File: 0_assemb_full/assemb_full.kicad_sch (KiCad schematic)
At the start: 19 parts, among them J1 BarrelJack, J11 OutToRPi, J2 Conn_02x06, J3 AudioJack3, J4 Servo0Conn_01x03, J5 Servo1Conn_01x03, J6 Servo2Conn_01x03, J7 Servo3Conn_01x03, J8 Servo4Conn_01x03, U1 LM2902, U2 LD1117S33TR_SOT223

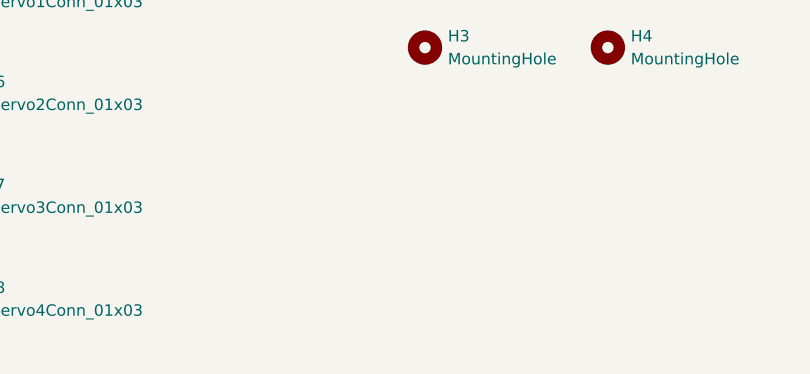
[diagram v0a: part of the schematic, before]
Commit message: Final adjustments
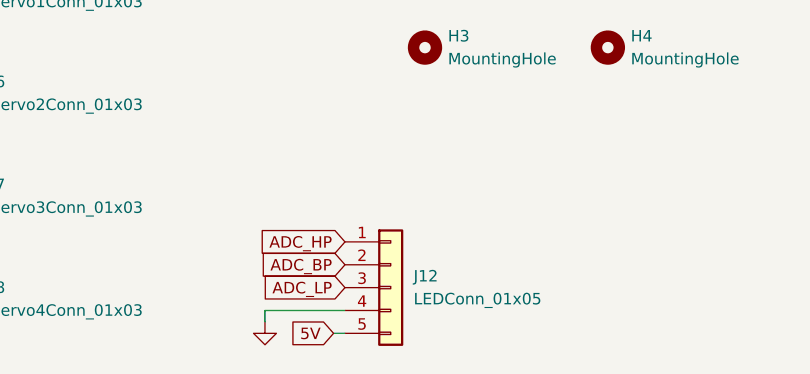
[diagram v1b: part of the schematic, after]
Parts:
- added J12: LEDConn_01x05, Connector_PinHeader_2.54mm:PinHeader_1x05_P2.54mm_Vertical, symbol Connector_Generic:Conn_01x05
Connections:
- net 5V: now also J12.5 (Pin_5)
- net GND: now also J12.4 (Pin_4)
- new net ADC_BP: J12.2 (Pin_2)
- new net ADC_HP: J12.1 (Pin_1)
- new net ADC_LP: J12.3 (Pin_3)
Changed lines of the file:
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@@
+    (stroke (width 0) (type default) (color 0 0 0 0))
+  )
+  (wire (pts (xy 68.58 191.77) (xy 59.69 191.77))
     (stroke (width 0) (type default) (color 0 0 0 0))
   )
@@
     (stroke (width 0) (type default) (color 0 0 0 0))
   )
+  (wire (pts (xy 59.69 191.77) (xy 59.69 193.04))
+    (stroke (width 0) (type default) (color 0 0 0 0))
+  )
   (wire (pts (xy 257.81 74.93) (xy 270.51 74.93))
     (stroke (width 0) (type default) (color 0 0 0 0))
@@
   )
   (wire (pts (xy 243.84 20.32) (xy 242.57 20.32))
+    (stroke (width 0) (type default) (color 0 0 0 0))
+  )
+  (wire (pts (xy 67.31 194.31) (xy 68.58 194.31))
     (stroke (width 0) (type default) (color 0 0 0 0))
   )
@@
   (text "Buck Connections" (at 236.22 53.34 0)
     (effects (font (size 1.27 1.27)) (justify left bottom))
+  )
+  (global_label "ADC_BP" (shape input) (at 68.58 186.69 180) (fields_autoplaced)
+    (effects (font (size 1.27 1.27)) (justify right))
+    (property "Intersheet References" "${INTERSHEET_REFS}" (id 0) (at 59.0307 186.6106 0)
+      (effects (font (size 1.27 1.27)) (justify right) hide)
+    )
+  )
+  (global_label "5V" (shape input) (at 67.31 194.31 180) (fields_autoplaced)
+    (effects (font (size 1.27 1.27)) (justify right))
+    (property "Intersheet References" "${INTERSHEET_REFS}" (id 0) (at 62.5988 194.2306 0)
+      (effects (font (size 1.27 1.27)) (justify right) hide)
+    )
   )
   (global_label "5V" (shape input) (at 21.59 179.07 180) (fields_autoplaced)
@@
     )
   )
+  (global_label "ADC_LP" (shape input) (at 68.58 189.23 180) (fields_autoplaced)
+    (effects (font (size 1.27 1.27)) (justify right))
+    (property "Intersheet References" "${INTERSHEET_REFS}" (id 0) (at 59.2726 189.1506 0)
+      (effects (font (size 1.27 1.27)) (justify right) hide)
+    )
+  )
   (global_label "5V" (shape input) (at 21.59 167.64 180) (fields_autoplaced)
     (effects (font (size 1.27 1.27)) (justify right))
@@
     (effects (font (size 1.27 1.27)) (justify right))
     (property "Intersheet References" "${INTERSHEET_REFS}" (id 0) (at 16.8788 156.1306 0)
+      (effects (font (size 1.27 1.27)) (justify right) hide)
+    )
+  )
+  (global_label "ADC_HP" (shape input) (at 68.58 184.15 180) (fields_autoplaced)
+    (effects (font (size 1.27 1.27)) (justify right))
+    (property "Intersheet References" "${INTERSHEET_REFS}" (id 0) (at 58.9702 184.0706 0)
       (effects (font (size 1.27 1.27)) (justify right) hide)
     )
@@
     (pin "3")
   )
+  (symbol (lib_id "Connector_Generic:Conn_01x05") (at 73.66 189.23 0) (unit 1)
+    (in_bom yes) (on_board yes) (fields_autoplaced)
+    (property "Reference" "J12" (id 0) (at 76.2 187.9599 0)
+      (effects (font (size 1.27 1.27)) (justify left))
+    )
+    (property "Value" "LEDConn_01x05" (id 1) (at 76.2 190.4999 0)
+      (effects (font (size 1.27 1.27)) (justify left))
+    )
+    (property "Footprint" "Connector_PinHeader_2.54mm:PinHeader_1x05_P2.54mm_Vertical" (id 2) (at 73.66 189.23 0)
+      (effects (font (size 1.27 1.27)) hide)
+    )
+    (property "Datasheet" "~" (id 3) (at 73.66 189.23 0)
+      (effects (font (size 1.27 1.27)) hide)
+    )
+    (pin "1")
+    (pin "2")
+    (pin "3")
+    (pin "4")
+    (pin "5")
+  )
   (symbol (lib_id "power:GND") (at 242.57 21.59 0) (unit 1)
     (in_bom yes) (on_board yes) (fields_autoplaced)
@@
     )
     (property "Datasheet" "" (id 3) (at 267.97 46.99 0)
+      (effects (font (size 1.27 1.27)) hide)
+    )
+    (pin "1")
+  )
+  (symbol (lib_id "power:GND") (at 59.69 193.04 0) (unit 1)
+    (in_bom yes) (on_board yes) (fields_autoplaced)
+    (property "Reference" "#PWR02" (id 0) (at 59.69 199.39 0)
+      (effects (font (size 1.27 1.27)) hide)
+    )
+    (property "Value" "GND" (id 1) (at 59.69 198.12 0)
+      (effects (font (size 1.27 1.27)) hide)
+    )
+    (property "Footprint" "" (id 2) (at 59.69 193.04 0)
+      (effects (font (size 1.27 1.27)) hide)
+    )
+    (property "Datasheet" "" (id 3) (at 59.69 193.04 0)
       (effects (font (size 1.27 1.27)) hide)
     )
@@
       (reference "#PWR01") (unit 1) (value "GND") (footprint "")
     )
+    (path "/5f6b1080-20a3-4632-95ab-7b720d91eec0"
+      (reference "#PWR02") (unit 1) (value "GND") (footprint "")
+    )
     (path "/5d07cb7e-c8e3-4ee6-8941-4590fa1e9acf"
       (reference "#PWR03") (unit 1) (value "GND") (footprint "")
@@
       (reference "J11") (unit 1) (value "OutToRPi") (footprint "Connector_PinHeader_2.54mm:PinHeader_1x02_P2.54mm_Vertical")
     )
+    (path "/1d0ef5db-c335-4d55-88dd-66a03b46c698"
+      (reference "J12") (unit 1) (value "LEDConn_01x05") (footprint "Connector_PinHeader_2.54mm:PinHeader_1x05_P2.54mm_Vertical")
+    )
+    (path "/4d0bd211-4794-4141-8b4c-fc5ed36fe38a/2faa9641-2ece-4171-8790-3945bf54da23"
+      (reference "J13") (unit 1) (value "RPiConn_01x03") (footprint "Connector_PinSocket_2.54mm:PinSocket_1x03_P2.54mm_Vertical")
+    )
     (path "/ba21e8b0-efb7-4c13-98e2-ebc8a39461f9"

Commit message: Final changes to PCB after footprint tests.
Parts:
- J1: footprint Connector_BarrelJack:BarrelJack_CUI_PJ-102AH_Horizontal -> Connector_BarrelJack:BarrelJack_GCT_DCJ200-10-A_Horizontal
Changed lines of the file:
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@@
       (effects (font (size 1.27 1.27)) (justify left))
     )
-    (property "Footprint" "Connector_BarrelJack:BarrelJack_CUI_PJ-102AH_Horizontal" (id 2) (at 248.92 17.78 0)
+    (property "Footprint" "Connector_BarrelJack:BarrelJack_GCT_DCJ200-10-A_Horizontal" (id 2) (at 248.92 17.78 0)
       (effects (font (size 1.27 1.27)) hide)
     )
@@
     )
     (path "/3e1ccb16-5496-4985-9aa9-d268c89cac5f"
-      (reference "J1") (unit 1) (value "BarrelJack") (footprint "Connector_BarrelJack:BarrelJack_CUI_PJ-102AH_Horizontal")
+      (reference "J1") (unit 1) (value "BarrelJack") (footprint "Connector_BarrelJack:BarrelJack_GCT_DCJ200-10-A_Horizontal")
     )
     (path "/9119ee79-ac43-4908-ba85-62b847bd6c6c"
